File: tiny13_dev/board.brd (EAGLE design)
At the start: 20 x 20 mm, 6 parts, among them IC1 TINY13V-10SSU, X1 SSW-103-02-G-D, X2 SSW-104-02-G-S, X3 SSW-104-02-G-S

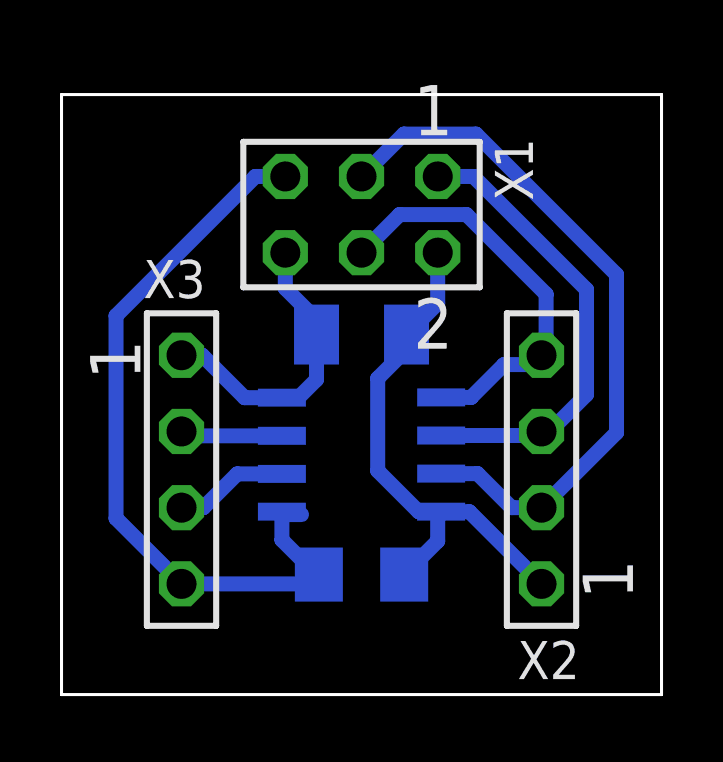
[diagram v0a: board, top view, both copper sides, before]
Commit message: optimized snowfall hw
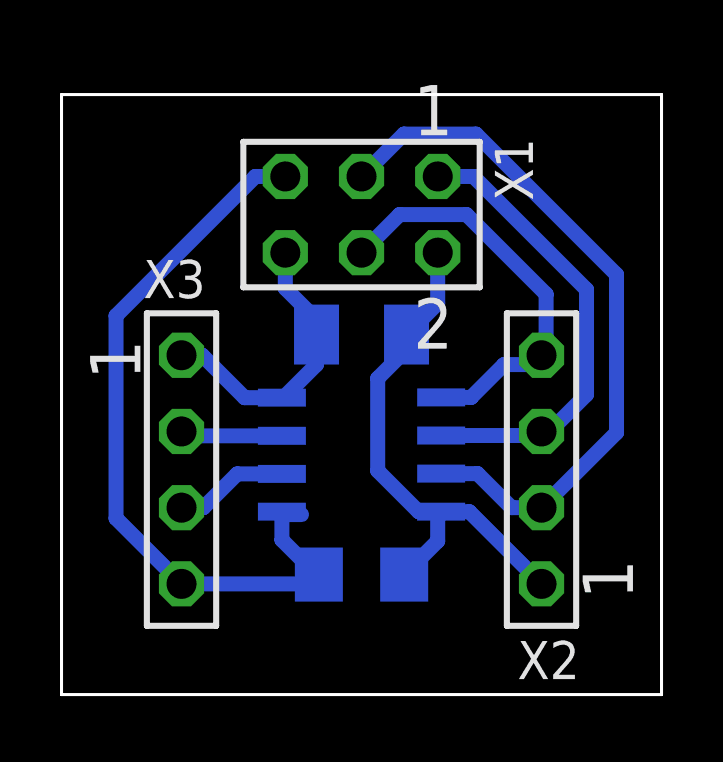
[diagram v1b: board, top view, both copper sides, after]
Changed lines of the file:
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@@
 <wire x1="15.46" y1="28.73" x2="15.46" y2="27.54" width="0.5" layer="16"/>
 <wire x1="16.615" y1="25.885" x2="16.5" y2="26" width="0.5" layer="16"/>
-<wire x1="16.5" y1="26" x2="16.5" y2="24.5" width="0.5" layer="16"/>
-<wire x1="15.346" y1="23.895" x2="15.895" y2="23.895" width="0.5" layer="16"/>
-<wire x1="16.5" y1="24.5" x2="15.895" y2="23.895" width="0.5" layer="16"/>
+<wire x1="16.5" y1="26" x2="16.5" y2="25" width="0.5" layer="16"/>
+<wire x1="15.346" y1="23.895" x2="15.395" y2="23.895" width="0.5" layer="16"/>
+<wire x1="16.5" y1="25" x2="15.395" y2="23.895" width="0.5" layer="16"/>
 <contactref element="X3" pad="1"/>
 <wire x1="12.69" y1="25.31" x2="12" y2="25.31" width="0.5" layer="16"/>
